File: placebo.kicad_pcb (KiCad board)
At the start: 2 copper layers, 19.1 x 29.2 mm, 14 parts, among them J1 ExtPower, J2 TagConnect, J3 Conn_01x10, J4 Conn_01x10, U1 AP7370-33W5-7, U2 STM32G0xxFx

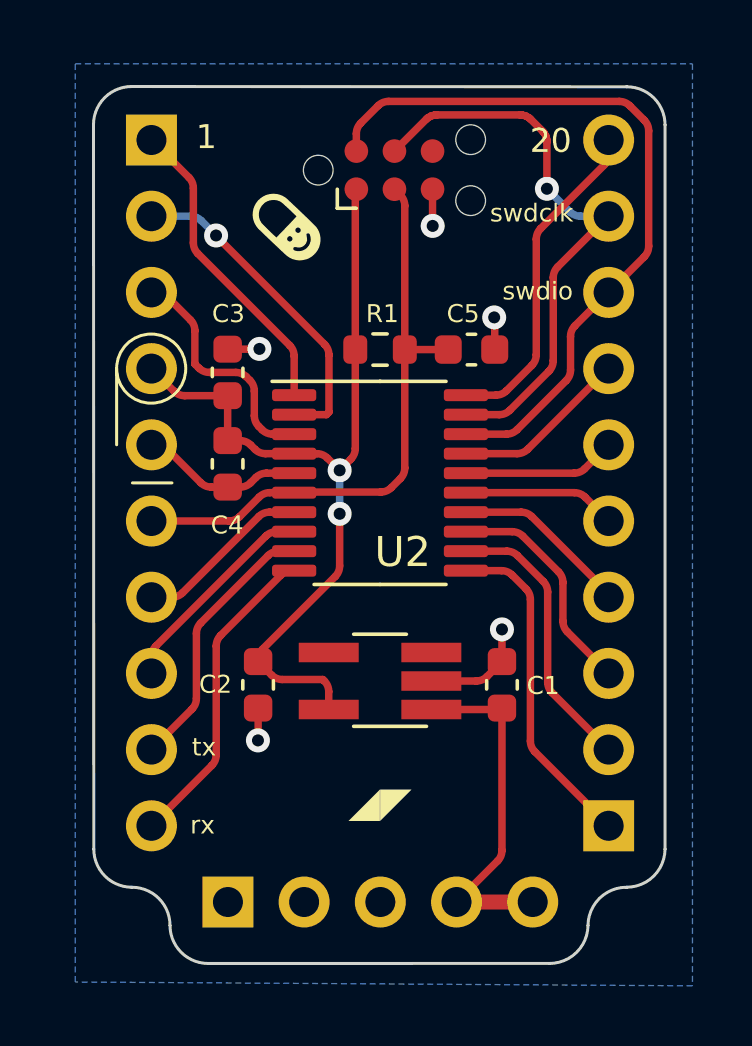
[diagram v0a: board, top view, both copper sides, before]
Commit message: PlaceboConnect
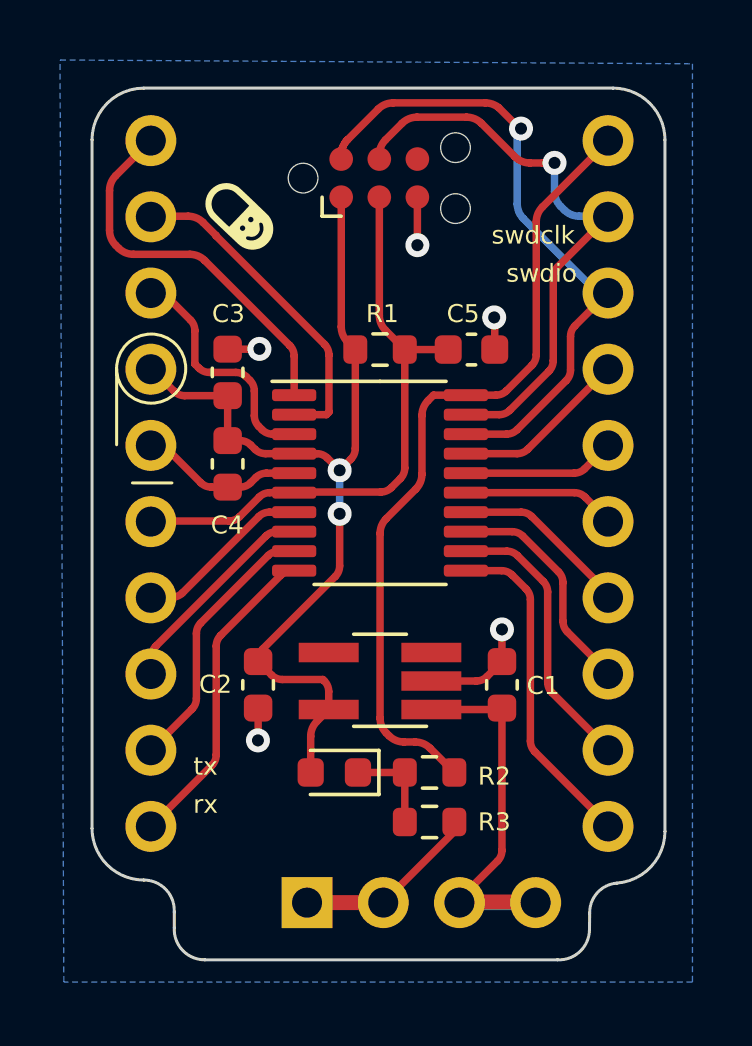
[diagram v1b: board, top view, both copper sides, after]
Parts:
- removed J1: ExtPower, Connector_PinHeader_2.54mm:PinHeader_1x05_P2.54mm_Vertical
- removed J3, J4: Conn_01x10, Connector_PinHeader_2.54mm:PinHeader_1x10_P2.54mm_Vertical
- removed the REF** at (74.3, 90.0)
- added D1: DNP, LED_SMD:LED_0603_1608Metric, F.Cu at (72.8, 104.4)
- added R2: DNP, Resistor_SMD:R_0603_1608Metric, F.Cu at (75.9, 104.4)
- added R3: DNP, Resistor_SMD:R_0603_1608Metric, F.Cu at (75.9, 106.0)
- added REF**: OSHW-Logo2_7.3x6mm_SilkScreen, Symbol:OSHW-Logo2_7.3x6mm_SilkScreen, B.Cu at (74.3, 90.0)
- added U3: PlaceboConnect, placebo:PlaceboConnect, F.Cu at (74.4, 94.7)
- moved G*** 1.61 mm to (69.6, 85.9)
- moved J2 0.57 mm to (74.3, 84.6)
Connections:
- net Net-(C1-Pad1) renamed VCC
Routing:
- net /PB3: track 11.1 -> 26.9 mm
- net GND: track 13.9 -> 20.8 mm
- net Net-(D1-K): track 0.00 -> 3.21 mm
- net VCC: track 11.8 -> 14.5 mm
- net /PB7: track 10.4 -> 12.9 mm
- net /SwdIO: track 24.8 -> 22.3 mm, vias 0 -> 1
- net +3V3: track 28.9 -> 31.1 mm
- net /SwdClk: track 19.3 -> 19.8 mm
- net /PB9: vias 1 -> 0
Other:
- board size 19.1 x 29.2 mm -> 19.1 x 29.1 mm
- board text added: "STM32G0xxFx Breakout rev. 0x5"
- board text removed: "1"
- board text removed: "20"
- board text removed: "STM32G0xxFx breakout rev. 0x4"
- board text removed: "◢◤"
